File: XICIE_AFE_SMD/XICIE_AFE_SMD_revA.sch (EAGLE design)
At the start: 26 parts, among them IC1 LM324D, IC2 CY8C4245T, IC3 AAT1217, J1 22-27-2031-03, Q1 MOSFET-NCHANNELBSS123LT1G, Q2 MOSFET-NCHANNELBSS123LT1G, Q3 MOSFET-NCHANNELBSS123LT1G

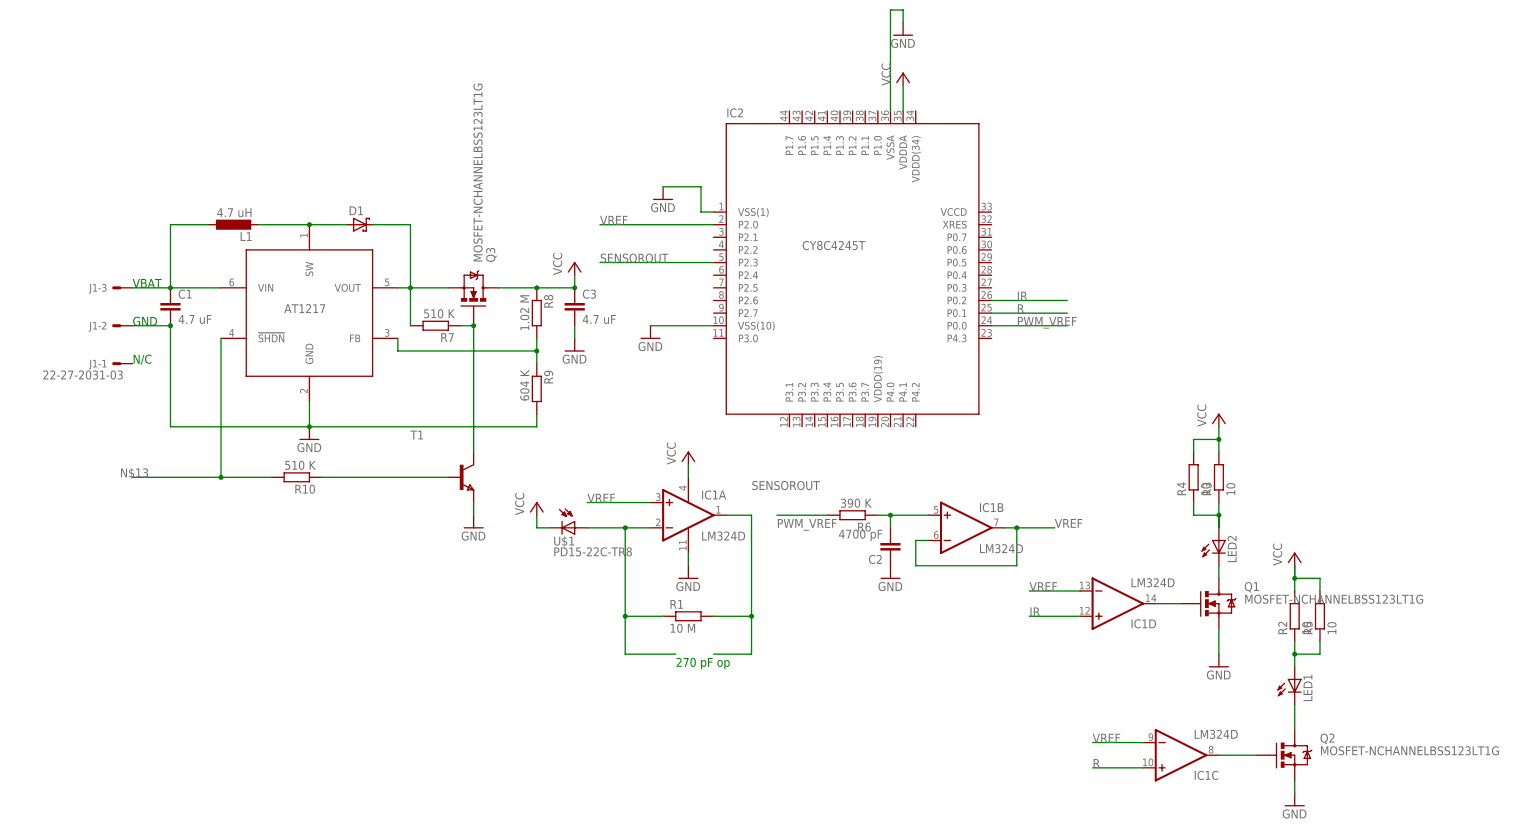
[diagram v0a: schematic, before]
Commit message: PCB Layoutd
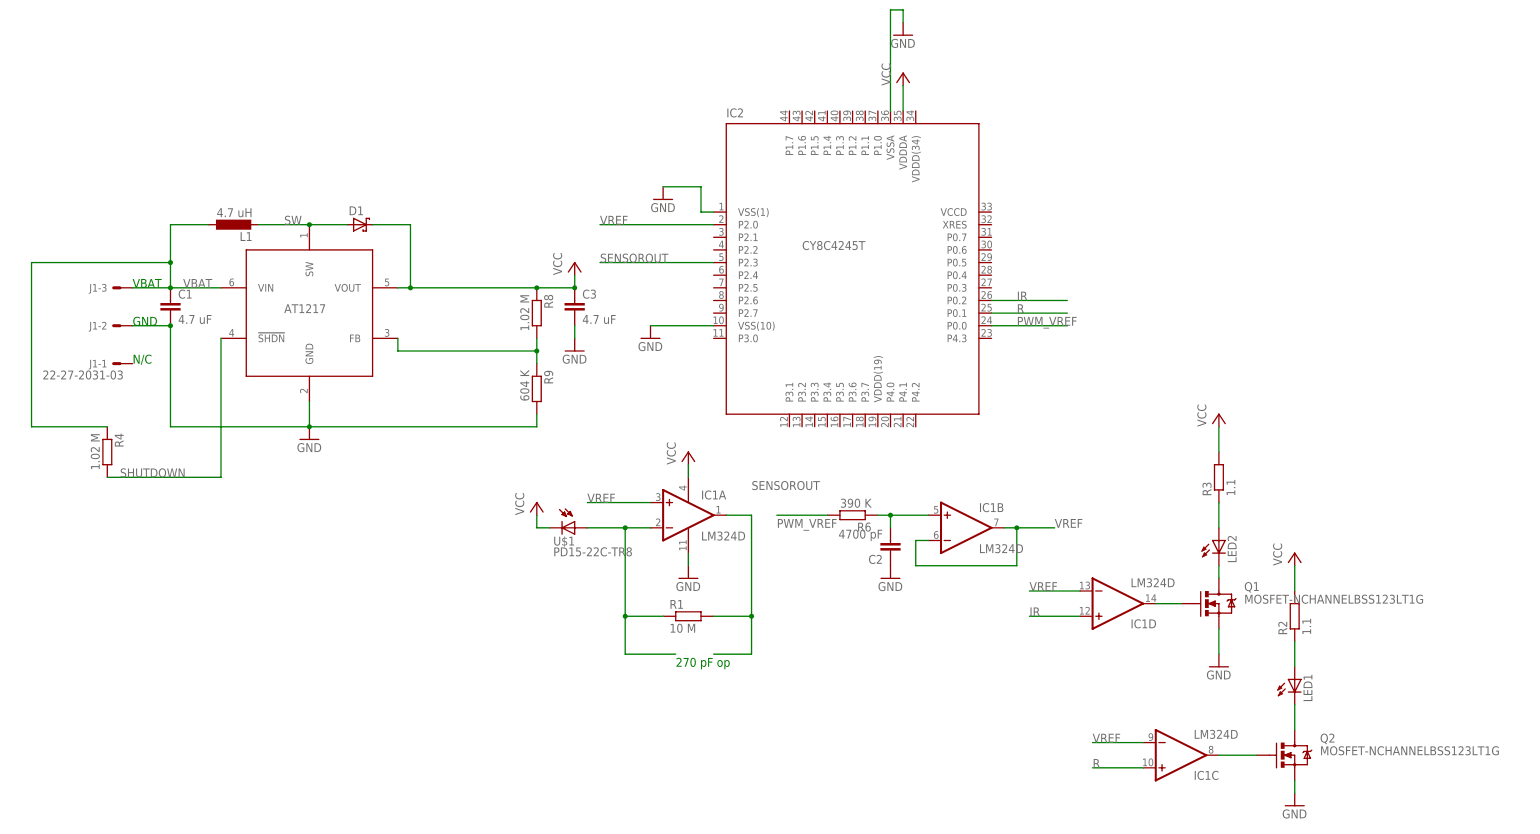
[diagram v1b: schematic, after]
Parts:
- removed Q3: MOSFET-NCHANNELBSS123LT1G, SparkFun-DiscreteSemi:MOSFET-NCHANNELBSS123LT1G
- removed R10, R7: 510 K, rcl:R-EU_R0603
- removed R5: 10, rcl:R-EU_R0603
- removed T1: (no value), zetex:NPNSOT23
- R2, R3: value 10 -> 1.1; device rcl:R-EU_R0603 -> rcl:R-EU_R0402
- R4: value 10 -> 1.02 M; device rcl:R-EU_R0603 -> rcl:R-EU_R0805
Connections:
- net N$2 renamed SW
- removed net N$10: C1.1, IC3.VIN, J1-3.S, L1.1
- removed net N$11: D1.C, IC3.VOUT, Q3.S, R7.2
- removed net N$12: Q3.G, R7.1, T1.C
- removed net N$13: IC3.!SHDN, R10.2
- removed net N$15: R10.1, T1.B
- new net SHUTDOWN: IC3.!SHDN, R4.2
- new net VBAT: C1.1, IC3.VIN, J1-3.S, L1.1, R4.1
- net GND: no longer T1.E
- net N$7: no longer R5.1
- net N$8: no longer R4.1
- net VCC: now also D1.C, IC3.VOUT; no longer Q3.D, R4.2, R5.2
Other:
- moved on the sheet: R4
